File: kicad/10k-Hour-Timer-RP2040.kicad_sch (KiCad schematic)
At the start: 15 parts, among them J1 Conn_01x03_Pin, J2 JST_SH_SM03B, J3 USB_C_Receptacle_USB2.0_16P, U1 USBLC6-2SC6

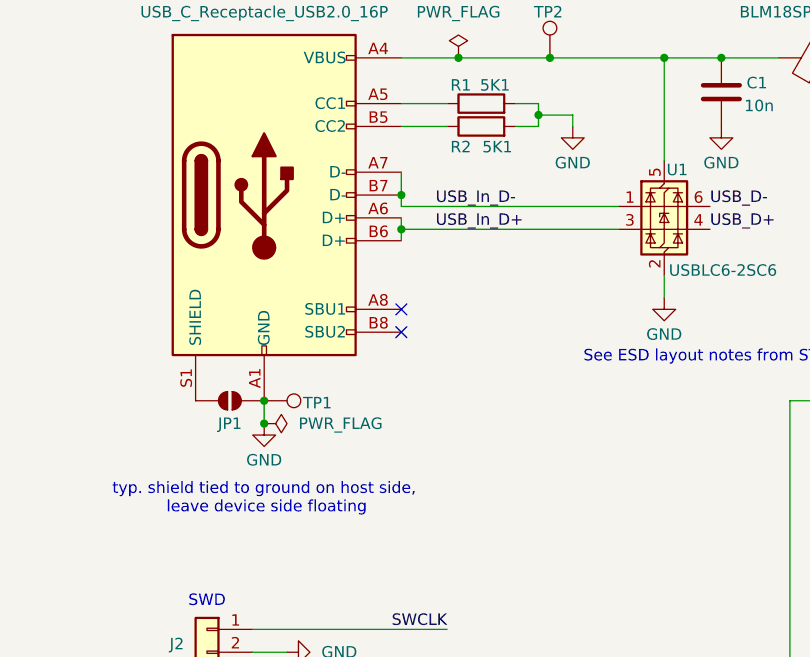
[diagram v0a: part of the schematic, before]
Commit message: floorplanning
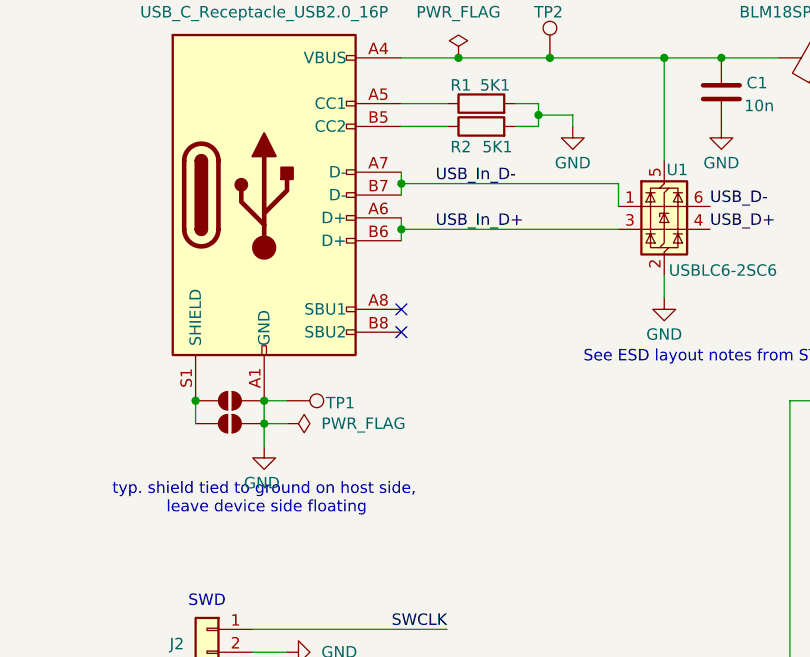
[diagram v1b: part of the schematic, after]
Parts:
- added JP24: SolderJumper_2_Open, Jumper:SolderJumper-2_P1.3mm_Open_RoundedPad1.0x1.5mm, symbol Jumper:SolderJumper_2_Open
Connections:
- net GND: now also JP24.2 (B)
- net at J3.S1 (SHIELD), JP1.1 (A): now also JP24.1 (A)
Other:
- moved on the sheet: TP1
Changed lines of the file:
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@@
 	)
 	(junction
-		(at 73.66 72.39)
+		(at 73.66 71.12)
 		(diameter 0)
 		(color 0 0 0 0)
@@
 	)
 	(junction
+		(at 50.8 95.25)
+		(diameter 0)
+		(color 0 0 0 0)
+	)
+	(junction
 		(at 58.42 95.25)
 		(diameter 0)
@@
 	(wire
 		(pts
+			(xy 60.96 95.25) (xy 58.42 95.25)
+		)
+		(stroke
+			(width 0)
+			(type default)
+		)
+	)
+	(wire
+		(pts
 			(xy 59.69 146.05) (xy 73.66 146.05)
 		)
@@
 	(wire
 		(pts
+			(xy 50.8 95.25) (xy 50.8 97.79)
+		)
+		(stroke
+			(width 0)
+			(type default)
+		)
+	)
+	(wire
+		(pts
 			(xy 210.82 147.32) (xy 184.15 147.32)
 		)
@@
 	(wire
 		(pts
+			(xy 58.42 100.33) (xy 58.42 97.79)
+		)
+		(stroke
+			(width 0)
+			(type default)
+		)
+	)
+	(wire
+		(pts
 			(xy 184.15 142.24) (xy 215.9 142.24)
 		)
@@
 	(wire
 		(pts
-			(xy 73.66 69.85) (xy 73.66 72.39)
+			(xy 73.66 69.85) (xy 73.66 71.12)
 		)
 		(stroke
@@
 	(wire
 		(pts
+			(xy 97.79 71.12) (xy 97.79 73.66)
+		)
+		(stroke
+			(width 0)
+			(type default)
+		)
+	)
+	(wire
+		(pts
 			(xy 123.19 57.15) (xy 125.73 57.15)
 		)
@@
 	(wire
 		(pts
+			(xy 60.96 97.79) (xy 58.42 97.79)
+		)
+		(stroke
+			(width 0)
+			(type default)
+		)
+	)
+	(wire
+		(pts
 			(xy 88.9 63.5) (xy 92.71 63.5)
 		)
@@
 	(wire
 		(pts
-			(xy 73.66 73.66) (xy 73.66 72.39)
+			(xy 73.66 71.12) (xy 73.66 72.39)
 		)
 		(stroke
@@
 	(wire
 		(pts
-			(xy 73.66 73.66) (xy 97.79 73.66)
+			(xy 73.66 71.12) (xy 97.79 71.12)
 		)
 		(stroke
@@
 	)
 	(label "USB_In_D-"
-		(at 77.47 73.66 0)
+		(at 77.47 71.12 0)
 		(effects
 			(font
@@
 					(size 1.27 1.27)
 				)
+				(hide yes)
 			)
 		)
@@
 	)
 	(symbol
+		(lib_id "Jumper:SolderJumper_2_Open")
+		(at 54.61 97.79 0)
+		(unit 1)
+		(exclude_from_sim no)
+		(in_bom no)
+		(on_board yes)
+		(dnp no)
+		(property "Reference" "JP24"
+			(at 54.61 100.33 0)
+			(effects
+				(font
+					(size 1.27 1.27)
+				)
+				(hide yes)
+			)
+		)
+		(property "Value" "SolderJumper_2_Open"
+			(at 39.624 103.124 0)
+			(effects
+				(font
+					(size 1.27 1.27)
+				)
+				(hide yes)
+			)
+		)
+		(property "Footprint" "Jumper:SolderJumper-2_P1.3mm_Open_RoundedPad1.0x1.5mm"
+			(at 54.61 97.79 0)
+			(effects
+				(font
+					(size 1.27 1.27)
+				)
+				(hide yes)
+			)
+		)
+		(property "Datasheet" "~"
+			(at 54.61 97.79 0)
+			(effects
+				(font
+					(size 1.27 1.27)
+				)
+				(hide yes)
+			)
+		)
+		(property "Description" "Solder Jumper, 2-pole, open"
+			(at 54.61 97.79 0)
+			(effects
+				(font
+					(size 1.27 1.27)
+				)
+				(hide yes)
+			)
+		)
+		(property "Subsystem" "01A-USB"
+			(at 54.61 97.79 0)
+			(effects
+				(font
+					(size 1.27 1.27)
+				)
+				(hide yes)
+			)
+		)
+		(property "MPN" "(Embedded)"
+			(at 54.61 97.79 0)
+			(effects
+				(font
+					(size 1.27 1.27)
+				)
+				(hide yes)
+			)
+		)
+		(pin "1"
+		)
+		(pin "2"
+		)
+		(instances
+			(project "10k-Hour-Timer-RP2040"
+				(path "/9d26b66f-2a94-42e5-8460-016e0bf95186"
+					(reference "JP24")
+					(unit 1)
+				)
+			)
+		)
+	)
+	(symbol
 		(lib_id "Connector:TestPoint")
 		(at 132.08 57.15 0)
@@
 	(symbol
 		(lib_id "Connector:TestPoint")
-		(at 58.42 95.25 270)
+		(at 60.96 95.25 270)
 		(unit 1)
 		(exclude_from_sim no)
@@
 		(dnp no)
 		(property "Reference" "TP1"
-			(at 62.738 95.504 90)
+			(at 65.278 95.504 90)
 			(effects
 				(font
@@
 		)
 		(property "Value" "GND"
-			(at 63.5 93.9801 90)
+			(at 66.04 93.9801 90)
 			(effects
 				(font
@@
 		)
 		(property "Footprint" "project footprints:TestPoint_THTPad_D2.0mm_Drill1.0mm"
-			(at 58.42 100.33 0)
+			(at 60.96 100.33 0)
 			(effects
 				(font
@@
 		)
 		(property "Datasheet" "~"
-			(at 58.42 100.33 0)
+			(at 60.96 100.33 0)
 			(effects
 				(font
@@
 		)
 		(property "Description" "test point"
-			(at 58.42 95.25 0)
+			(at 60.96 95.25 0)
 			(effects
 				(font
@@
 		)
 		(property "Subsystem" "01A-USB"
-			(at 58.42 95.25 90)
+			(at 60.96 95.25 90)
 			(effects
 				(font
@@
 		)
 		(property "MPN" "(Embedded)"
-			(at 58.42 95.25 90)
+			(at 60.96 95.25 90)
 			(effects
 				(font
@@
 	(symbol
 		(lib_id "power:PWR_FLAG")
-		(at 58.42 97.79 270)
+		(at 60.96 97.79 270)
 		(unit 1)
 		(exclude_from_sim no)
@@
 		(fields_autoplaced yes)
 		(property "Reference" "#FLG02"
-			(at 60.325 97.79 0)
+			(at 62.865 97.79 0)
 			(effects
 				(font
@@
 		)
 		(property "Value" "PWR_FLAG"
-			(at 62.23 97.7899 90)
+			(at 64.77 97.7899 90)
 			(effects
 				(font
@@
 		)
 		(property "Footprint" ""
-			(at 58.42 97.79 0)
+			(at 60.96 97.79 0)
 			(effects
 				(font
@@
 		)
 		(property "Datasheet" "~"
-			(at 58.42 97.79 0)
+			(at 60.96 97.79 0)
 			(effects
 				(font
@@
 		)
 		(property "Description" "Special symbol for telling ERC where power comes from"
-			(at 58.42 97.79 0)
+			(at 60.96 97.79 0)
 			(effects
 				(font
@@
 	(symbol
 		(lib_id "power:GND")
-		(at 58.42 97.79 0)
+		(at 58.42 100.33 0)
 		(unit 1)
 		(exclude_from_sim no)
@@
 		(dnp no)
 		(property "Reference" "#PWR03"
-			(at 58.42 104.14 0)
+			(at 58.42 106.68 0)
 			(effects
 				(font
@@
 		)
 		(property "Value" "GND"
-			(at 58.42 101.854 0)
+			(at 58.166 104.394 0)
 			(effects
 				(font
@@
 		)
 		(property "Footprint" ""
-			(at 58.42 97.79 0)
+			(at 58.42 100.33 0)
 			(effects
 				(font
@@
 		)
 		(property "Datasheet" ""
-			(at 58.42 97.79 0)
+			(at 58.42 100.33 0)
 			(effects
 				(font
@@
 		)
 		(property "Description" "Power symbol creates a global label with name \"GND\" , ground"
-			(at 58.42 97.79 0)
+			(at 58.42 100.33 0)
 			(effects
 				(font

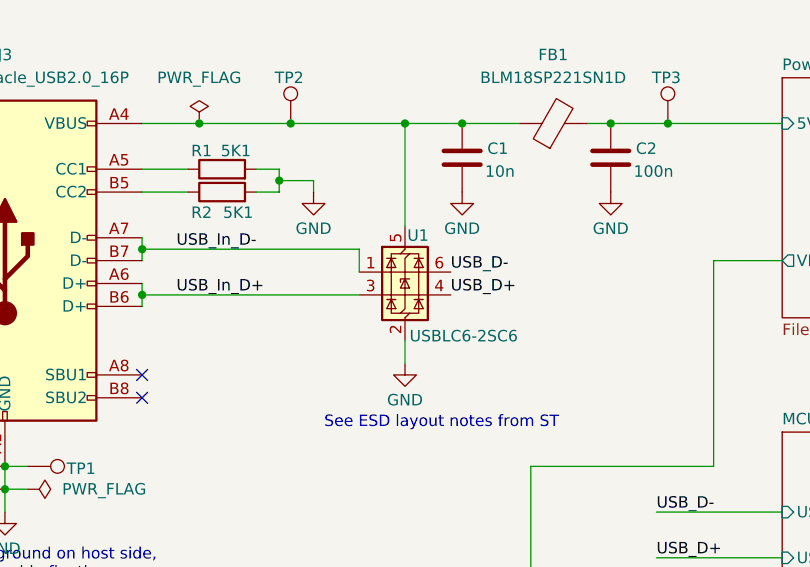
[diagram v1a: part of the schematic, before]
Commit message: buzzer fp, power mux layout
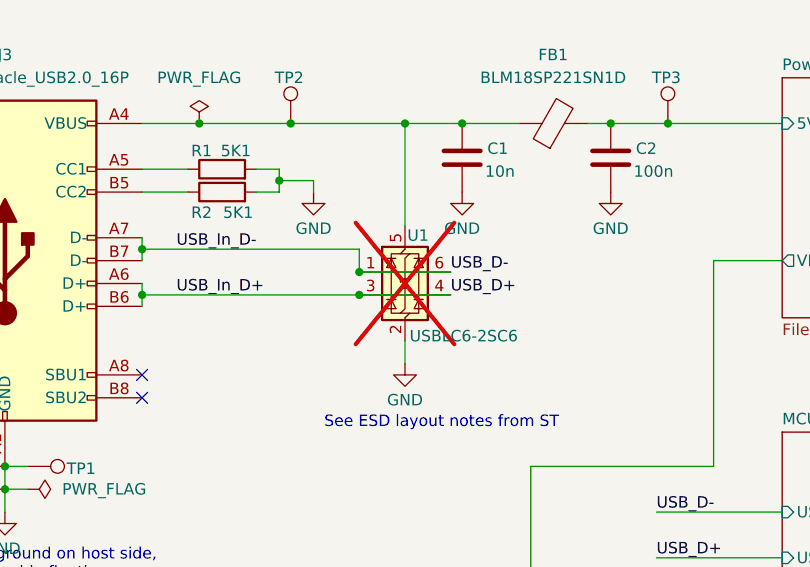
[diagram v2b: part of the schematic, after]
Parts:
- U1: now not fitted; now left out of the parts list
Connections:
- net USB_In_D+ is gone; now on net USB_D+: J3.A6 (D+), J3.B6 (D+), U1.3 (I/O2)
- net USB_In_D- is gone; now on net USB_D-: J3.A7 (D-), J3.B7 (D-), U1.1 (I/O1)
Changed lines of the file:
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@@
+	)
+	(junction
+		(at 97.79 76.2)
+		(diameter 0)
+		(color 0 0 0 0)
 	)
 	(junction
@@
 		(color 0 0 0 0)
 	)
+	(junction
+		(at 97.79 73.66)
+		(diameter 0)
+		(color 0 0 0 0)
+	)
 	(no_connect
 		(at 73.66 87.63)
@@
 	(wire
 		(pts
+			(xy 97.79 76.2) (xy 107.95 76.2)
+		)
+		(stroke
+			(width 0)
+			(type default)
+		)
+	)
+	(wire
+		(pts
 			(xy 210.82 62.23) (xy 210.82 101.6)
 		)
@@
 		(pts
 			(xy 60.96 97.79) (xy 58.42 97.79)
+		)
+		(stroke
+			(width 0)
+			(type default)
+		)
+	)
+	(wire
+		(pts
+			(xy 97.79 73.66) (xy 107.95 73.66)
 		)
 		(stroke
@@
 		(unit 1)
 		(exclude_from_sim no)
-		(in_bom yes)
-		(on_board yes)
-		(dnp no)
+		(in_bom no)
+		(on_board no)
+		(dnp yes)
 		(property "Reference" "U1"
 			(at 103.124 69.596 0)
